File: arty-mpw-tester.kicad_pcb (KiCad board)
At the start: 4 copper layers, 53.3 x 61.5 mm, 174 parts, among them J1 USB4105-GF-A, J10 61300211121, J11 61300211121, J12 61300211121, J14 61300311121, J15 61300311121, J18 61300411121, J19 61300711121, J20 61300411121, J3 arty_chipKIT_connector, J4 61300211121, J5 61300311121, J6 61300211121, J7 61300211121, J8 61300211121, J9 61300211121, Q1 DTC014TEBTL, SW1 JS202011JCQN, SW3 JS202011JCQN, U1 PAC1954T-E/4MX, U10 TPD4E02B04DQA, U11 TAR5S33UTE85LF, U2 FT4232H-56Q, U3 PAC1954T-E/4MX, U4 MAX811REUS+T, U5 NTS0102DP, U6 MCP4661-103E/ML, U7 Caravel_breakout_PCB_flexypin, U8 W25Q32FVSS, U9 MIC2211-AAYML-TR, Y1 ABM8G-12.000MHZ-18-D2Y-T, Y2 ECS-2520MVLC-100-BN-TR

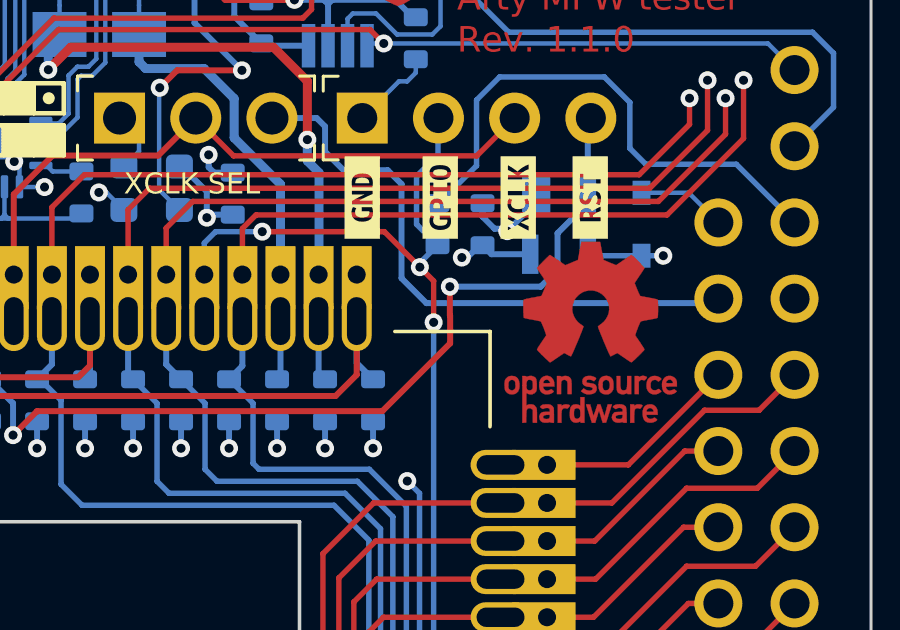
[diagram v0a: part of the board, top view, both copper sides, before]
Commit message: Added slight visual adjustments
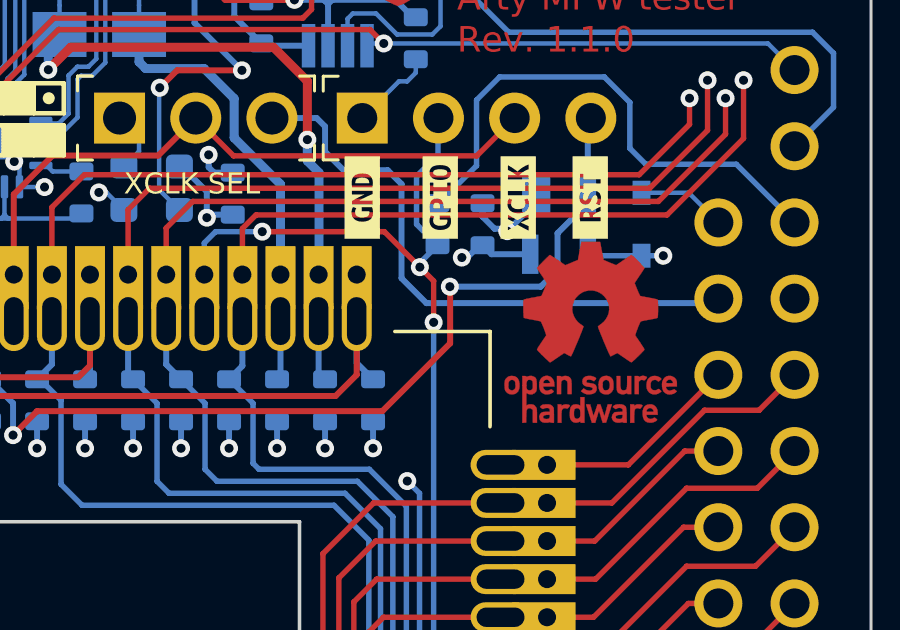
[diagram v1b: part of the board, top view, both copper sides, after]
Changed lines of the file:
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@@
   (segment (start 143.6 117.12) (end 140.8675 117.12) (width 0.15) (layer "B.Cu") (net 53))
   (segment (start 146.505 84.578) (end 146.505 86.128) (width 0.2) (layer "F.Cu") (net 54))
+  (segment (start 162.3105 84.9805) (end 162.32 84.99) (width 0.2) (layer "F.Cu") (net 54))
+  (segment (start 148.55 89.13) (end 147.75 89.93) (width 0.2) (layer "F.Cu") (net 54))
+  (segment (start 162.32 84.99) (end 162.32 86.87) (width 0.2) (layer "F.Cu") (net 54))
+  (segment (start 160.06 89.13) (end 148.55 89.13) (width 0.2) (layer "F.Cu") (net 54))
   (segment (start 162.32 86.87) (end 160.06 89.13) (width 0.2) (layer "F.Cu") (net 54))
-  (segment (start 160.06 89.13) (end 148.55 89.13) (width 0.2) (layer "F.Cu") (net 54))
-  (segment (start 148.55 89.13) (end 147.75 89.93) (width 0.2) (layer "F.Cu") (net 54))
-  (segment (start 162.32 85.942182) (end 162.32 86.87) (width 0.2) (layer "F.Cu") (net 54))
-  (segment (start 162.3105 84.9805) (end 162.3105 85.932682) (width 0.2) (layer "F.Cu") (net 54))
-  (segment (start 162.3105 85.932682) (end 162.32 85.942182) (width 0.2) (layer "F.Cu") (net 54))
   (via (at 162.3105 84.9805) (size 0.6) (drill 0.3) (layers "F.Cu" "B.Cu") (net 54))
   (via (at 147.75 89.93) (size 0.6) (drill 0.3) (layers "F.Cu" "B.Cu") (net 54))

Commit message: Loclib
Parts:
- C8: footprint antmicro-footprints:0603-cap -> arty-mpw-tester-footprints:0603-cap
- FB1, FB2, FB3: footprint antmicro-footprints:0603-res -> arty-mpw-tester-footprints:0603-res
- NT1, NT10, NT11, NT12, NT13, NT14, NT2, NT3, NT4, NT5, NT6, NT7, NT8, NT9: footprint antmicro-footprints:NetTie-2_SMD_Pad0.15mm -> arty-mpw-tester-footprints:NetTie-2_SMD_Pad0.15mm
- R1, R10, R38, R39, R40, R41, R9: footprint antmicro-footprints:1206-res -> arty-mpw-tester-footprints:1206-res
- U1, U3: footprint antmicro-footprints:VQFN-16-1EP_3x3mm_P0.5mm_EP1.1x1.1mm -> arty-mpw-tester-footprints:VQFN-16-1EP_3x3mm_P0.5mm_EP1.1x1.1mm
- U11: footprint antmicro-footprints:SOT-353 -> arty-mpw-tester-footprints:SOT-353
- U2: footprint antmicro-footprints:QFN-56-1EP_8x8mm_P0.5mm_EP5.5.9x5.9mm -> arty-mpw-tester-footprints:QFN-56-1EP_8x8mm_P0.5mm_EP5.5.9x5.9mm
